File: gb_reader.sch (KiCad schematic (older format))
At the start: 52 parts, among them J1 Conn_01x32_MountingPin, J2 USB_B_Micro, J3 Conn_01x09, J4 Conn_01x04, J5 Conn_01x32, SW0 SW, SW1 SW, SW2 SW, SW3 SW, U1 STM32F103RFTx, U2 TXB0108DQSR, U3 TXB0108DQSR, U4 TXB0108DQSR, U5 TXB0108DQSR, U6 LM317_3PinPackage, Y1 Crystal_Small

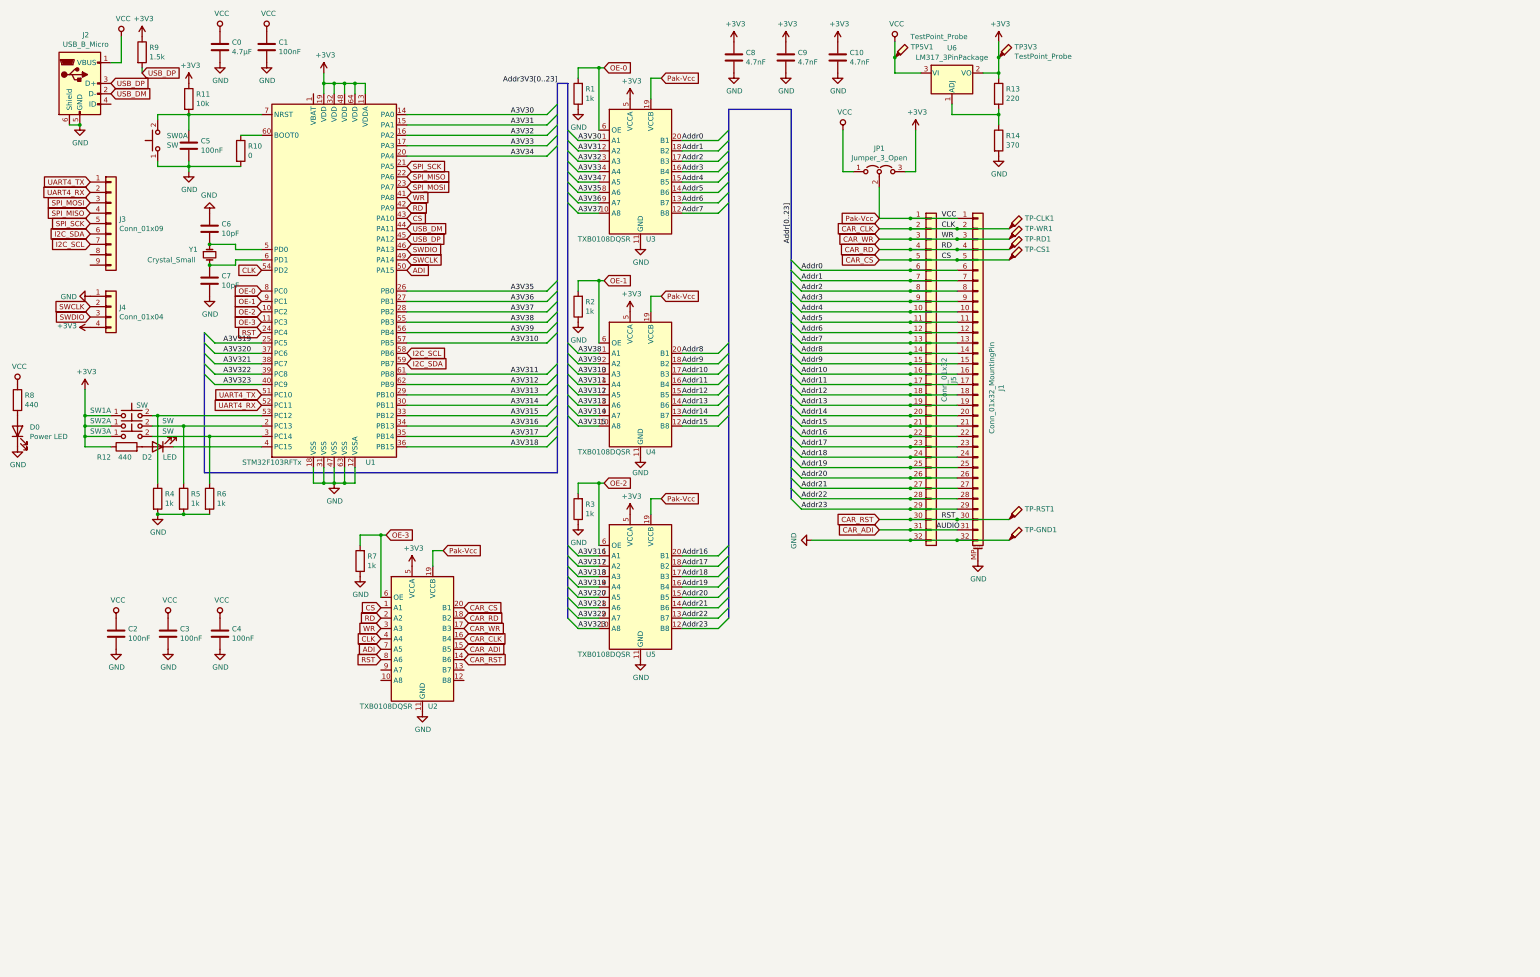
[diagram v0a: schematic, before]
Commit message: pcb layouting
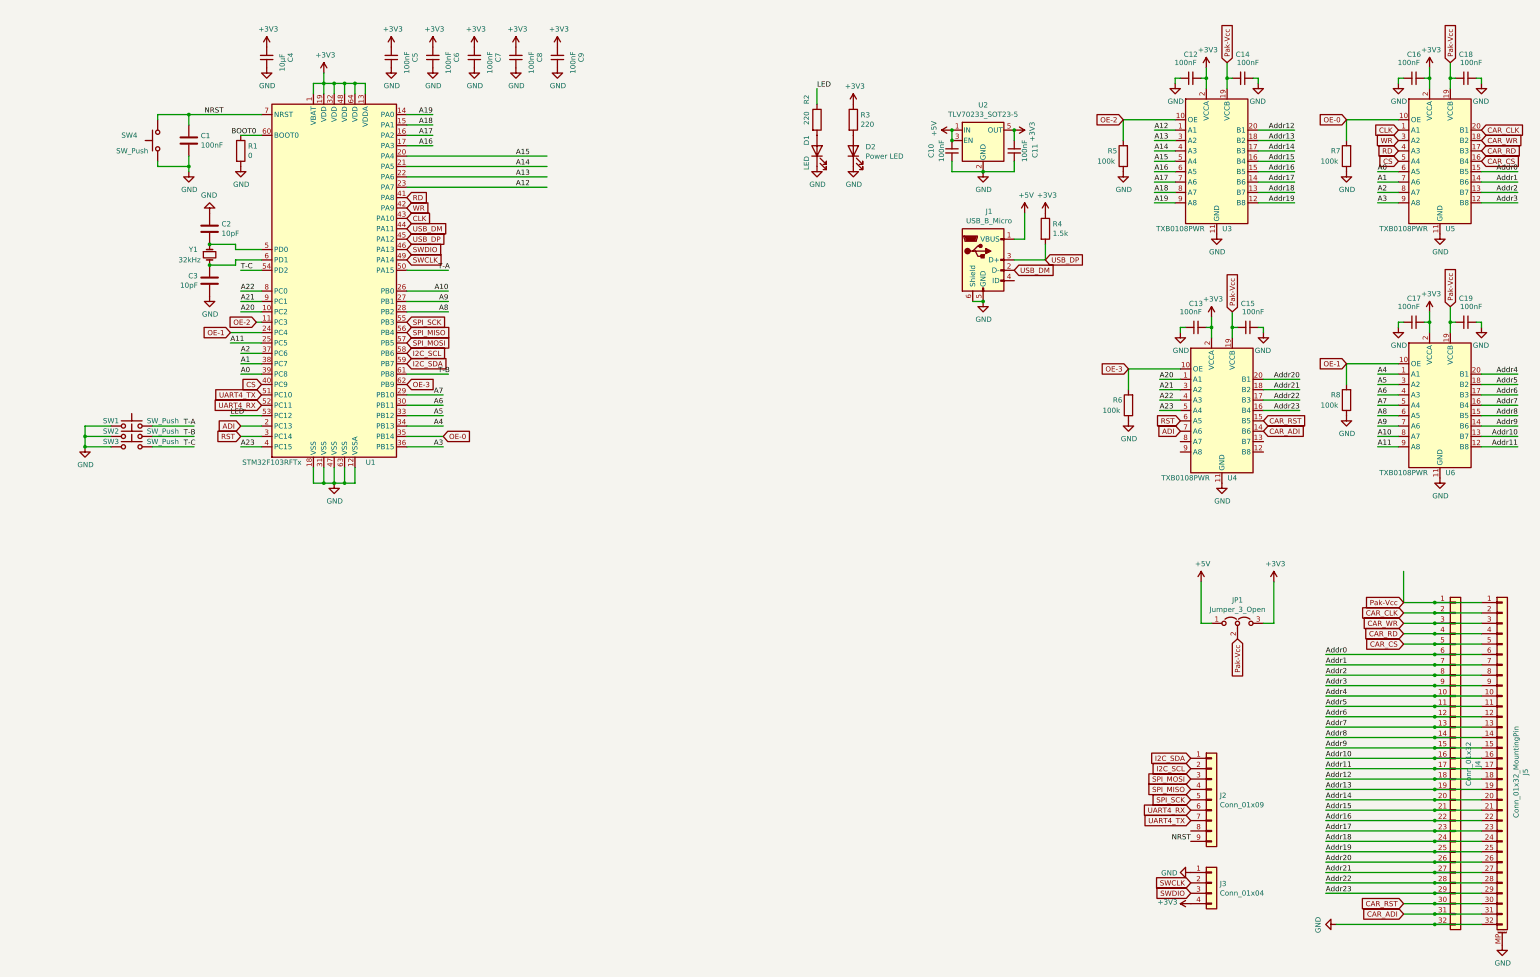
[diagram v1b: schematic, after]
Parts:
- removed C0: 4.7µF, Capacitor_SMD:C_0805_2012Metric, symbol Device:C
- removed C1, C2, C3, C4: 100nF, Capacitor_SMD:C_0603_1608Metric, symbol Device:C
- removed C10, C8, C9: 4.7nF, Capacitor_SMD:C_0603_1608Metric, symbol Device:C
- removed R1, R2, R3, R4: 1k, Resistor_SMD:R_0603_1608Metric, symbol Device:R
- removed R11: 10k, Resistor_SMD:R_0603_1608Metric, symbol Device:R
- removed R13: 220, Resistor_SMD:R_0603_1608Metric, symbol Device:R
- removed R14: 370, Resistor_SMD:R_0603_1608Metric, symbol Device:R
- removed SW0, SW1, SW2, SW3: SW, Button_Switch_THT:SW_TH_Tactile_Omron_B3F-10xx, symbol Switch:SW_Push_Dual_x2
- removed TP-CLK1, TP-CS1, TP-GND1, TP-RD1, TP-RST1, TP-WR1: (no value), TestPoint:TestPoint_Pad_D2.0mm, symbol Connector:TestPoint_Probe
- removed TP3V3, TP5V1: TestPoint_Probe, TestPoint:TestPoint_Pad_D2.0mm, symbol Connector:TestPoint_Probe
- removed U2, U3, U4, U5: TXB0108DQSR, Package_SON:USON-20_2x4mm_P0.4mm, symbol Logic_LevelTranslator:TXB0108DQSR
- removed U6: LM317_3PinPackage, Package_TO_SOT_SMD:SOT-223-3_TabPin2, symbol Regulator_Linear:LM317_3PinPackage
- added C10, C11, C12, C13, C14, C15, C16, C17, C18, C19, C5, C6, C7, C8, C9: 100nF, Capacitor_SMD:C_0603_1608Metric, symbol Device:C_Small
- added C4: 10µF, Capacitor_SMD:C_0603_1608Metric, symbol Device:C_Small
- added R8: 100k, Resistor_SMD:R_0603_1608Metric, symbol Device:R
- added SW1, SW2, SW3, SW4: SW_Push, Button_Switch_SMD:SW_Push_1P1T_NO_CK_KMR2, symbol Switch:SW_Push
- added U2: TLV70233_SOT23-5, Package_TO_SOT_SMD:SOT-23-5, symbol Regulator_Linear:TLV70233_SOT23-5
- added U3, U4, U5, U6: TXB0108PWR, Package_SO:TSSOP-20_4.4x6.5mm_P0.65mm, symbol Logic_LevelTranslator:TXB0108PWR
- J4: renamed from J5; footprint Connector_PinHeader_2.54mm:PinHeader_1x32_P2.54mm_Horizontal -> Connector_PinHeader_2.54mm:PinHeader_1x32_P2.54mm_Vertical
- JP1: footprint (none) -> Connector_PinHeader_2.54mm:PinHeader_1x03_P2.54mm_Vertical
- R2: renamed from R12; value 440 -> 220
- R3: renamed from R8; value 440 -> 220
- R5, R6, R7: value 1k -> 100k
- Y1: value Crystal_Small -> 32kHz
- renumbered C5 to C1, C6 to C2, C7 to C3, D2 to D1, D0 to D2, J2 to J1, J3 to J2, J4 to J3, J1 to J5, R10 to R1, R9 to R4
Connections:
- net labels added: +5V, A0, A1, A10, A11, A12, A13, A14, A15, A16, A17, A18, A19, A2, A20, A21, A22, A23, A3, A4, A5, A6, A7, A8, A9, BOOT0, LED, NRST, T-A, T-B, T-C
- net labels removed: A3V30, A3V31, A3V310, A3V311, A3V312, A3V313, A3V314, A3V315, A3V316, A3V317, A3V318, A3V319, A3V32, A3V320, A3V321, A3V322, A3V323, A3V33, A3V34, A3V35, A3V36, A3V37, A3V38, A3V39, AUDIO, Addr3V3[0..23], Addr[0..23], VCC
- wire segments 241 -> 254
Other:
- moved on the sheet: C1, D1, D2, J1, J2, J3, J4, J5, JP1, R2, R3, R4
